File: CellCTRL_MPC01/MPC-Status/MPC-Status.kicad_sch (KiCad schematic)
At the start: 38 parts, among them J1 Programming, J2 I2C, J3 Reset, U1 ATtiny202-SS

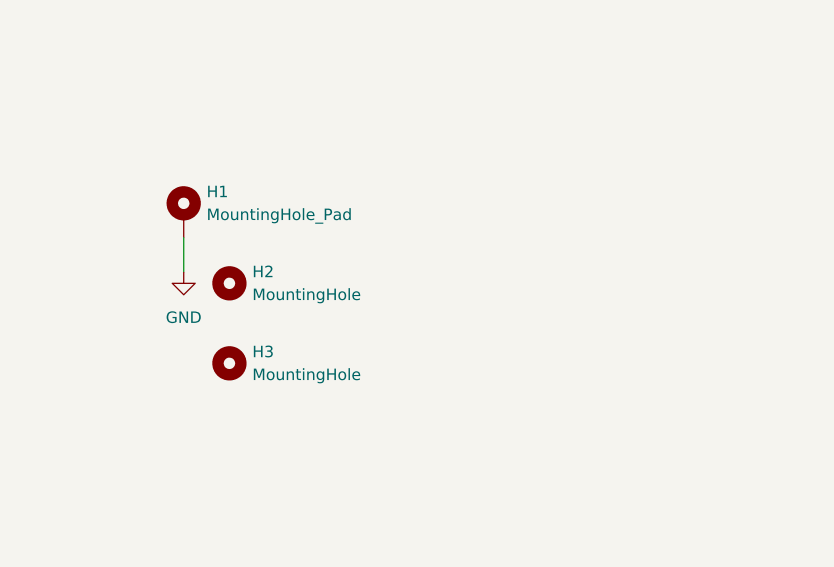
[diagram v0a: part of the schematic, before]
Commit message: Fertig V0.1_Status
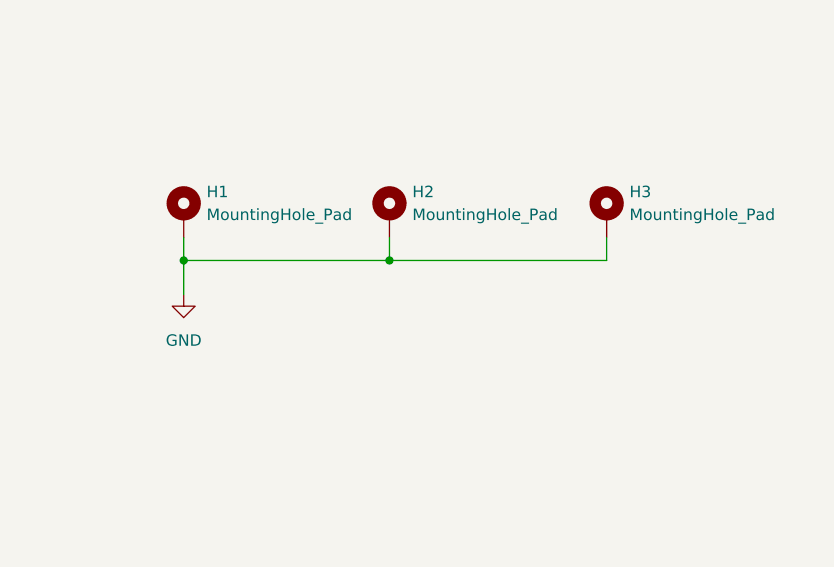
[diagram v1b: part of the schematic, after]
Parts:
- removed H2, H3: MountingHole, MountingHole:MountingHole_3.2mm_M3_DIN965, symbol Mechanical:MountingHole
- added H2, H3: MountingHole_Pad, MountingHole:MountingHole_3.2mm_M3_DIN965_Pad, symbol Mechanical:MountingHole_Pad
- J2: footprint Connector_JST:JST_EH_B4B-EH-A_1x04_P2.50mm_Vertical -> Connector_JST:JST_XH_B4B-XH-A_1x04_P2.50mm_Vertical
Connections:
- net GND: now also H2.1, H3.1
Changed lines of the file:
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@@
 	)
 	(junction
+		(at 227.33 93.98)
+		(diameter 0)
+		(color 0 0 0 0)
+	)
+	(junction
 		(at 82.55 148.59)
 		(diameter 0)
@@
 	)
 	(junction
+		(at 204.47 93.98)
+		(diameter 0)
+		(color 0 0 0 0)
+	)
+	(junction
 		(at 152.4 34.29)
 		(diameter 0)
@@
 	(wire
 		(pts
+			(xy 251.46 93.98) (xy 227.33 93.98)
+		)
+		(stroke
+			(width 0)
+			(type default)
+		)
+	)
+	(wire
+		(pts
 			(xy 57.15 135.89) (xy 62.23 135.89)
 		)
@@
 	(wire
 		(pts
+			(xy 251.46 91.44) (xy 251.46 93.98)
+		)
+		(stroke
+			(width 0)
+			(type default)
+		)
+	)
+	(wire
+		(pts
 			(xy 62.23 133.35) (xy 62.23 135.89)
 		)
@@
 	(wire
 		(pts
+			(xy 227.33 93.98) (xy 204.47 93.98)
+		)
+		(stroke
+			(width 0)
+			(type default)
+		)
+	)
+	(wire
+		(pts
 			(xy 160.02 46.99) (xy 167.64 46.99)
 		)
@@
 	(wire
 		(pts
-			(xy 204.47 91.44) (xy 204.47 95.25)
+			(xy 227.33 91.44) (xy 227.33 93.98)
+		)
+		(stroke
+			(width 0)
+			(type default)
+		)
+	)
+	(wire
+		(pts
+			(xy 204.47 91.44) (xy 204.47 93.98)
 		)
 		(stroke
@@
 	(wire
 		(pts
+			(xy 204.47 93.98) (xy 204.47 97.79)
+		)
+		(stroke
+			(width 0)
+			(type default)
+		)
+	)
+	(wire
+		(pts
 			(xy 198.12 39.37) (xy 198.12 34.29)
 		)
@@
 	)
 	(symbol
-		(lib_id "Mechanical:MountingHole")
-		(at 209.55 105.41 0)
-		(unit 1)
-		(exclude_from_sim no)
-		(in_bom no)
-		(on_board yes)
-		(dnp no)
-		(fields_autoplaced yes)
-		(property "Reference" "H3"
-			(at 212.09 104.1399 0)
-			(effects
-				(font
-					(size 1.27 1.27)
-				)
-				(justify left)
-			)
-		)
-		(property "Value" "MountingHole"
-			(at 212.09 106.6799 0)
-			(effects
-				(font
-					(size 1.27 1.27)
-				)
-				(justify left)
-			)
-		)
-		(property "Footprint" "MountingHole:MountingHole_3.2mm_M3_DIN965"
-			(at 209.55 105.41 0)
-			(effects
-				(font
-					(size 1.27 1.27)
-				)
-				(hide yes)
-			)
-		)
-		(property "Datasheet" "~"
-			(at 209.55 105.41 0)
-			(effects
-				(font
-					(size 1.27 1.27)
-				)
-				(hide yes)
-			)
-		)
-		(property "Description" "Mounting Hole without connection"
-			(at 209.55 105.41 0)
-			(effects
-				(font
-					(size 1.27 1.27)
-				)
-				(hide yes)
-			)
-		)
-		(instances
-			(project "MPC-Status"
-				(path "/6205391b-a61f-4e60-b73e-3eadab0d3997"
-					(reference "H3")
-					(unit 1)
-				)
-			)
-		)
-	)
-	(symbol
 		(lib_id "power:GND")
 		(at 152.4 20.32 180)
@@
 	)
 	(symbol
-		(lib_id "Mechanical:MountingHole")
-		(at 209.55 96.52 0)
-		(unit 1)
-		(exclude_from_sim no)
-		(in_bom no)
-		(on_board yes)
-		(dnp no)
-		(fields_autoplaced yes)
-		(property "Reference" "H2"
-			(at 212.09 95.2499 0)
-			(effects
-				(font
-					(size 1.27 1.27)
-				)
-				(justify left)
-			)
-		)
-		(property "Value" "MountingHole"
-			(at 212.09 97.7899 0)
-			(effects
-				(font
-					(size 1.27 1.27)
-				)
-				(justify left)
-			)
-		)
-		(property "Footprint" "MountingHole:MountingHole_3.2mm_M3_DIN965"
-			(at 209.55 96.52 0)
-			(effects
-				(font
-					(size 1.27 1.27)
-				)
-				(hide yes)
-			)
-		)
-		(property "Datasheet" "~"
-			(at 209.55 96.52 0)
-			(effects
-				(font
-					(size 1.27 1.27)
-				)
-				(hide yes)
-			)
-		)
-		(property "Description" "Mounting Hole without connection"
-			(at 209.55 96.52 0)
-			(effects
-				(font
-					(size 1.27 1.27)
-				)
-				(hide yes)
-			)
-		)
-		(instances
-			(project ""
-				(path "/6205391b-a61f-4e60-b73e-3eadab0d3997"
-					(reference "H2")
-					(unit 1)
-				)
-			)
-		)
-	)
-	(symbol
 		(lib_id "Device:C")
 		(at 175.26 26.67 180)
@@
 	(symbol
 		(lib_id "power:GND")
-		(at 204.47 95.25 0)
+		(at 204.47 97.79 0)
 		(unit 1)
 		(exclude_from_sim no)
@@
 		(fields_autoplaced yes)
 		(property "Reference" "#PWR030"
-			(at 204.47 101.6 0)
+			(at 204.47 104.14 0)
 			(effects
 				(font
@@
 		)
 		(property "Value" "GND"
-			(at 204.47 100.33 0)
+			(at 204.47 102.87 0)
 			(effects
 				(font
@@
 		)
 		(property "Footprint" ""
-			(at 204.47 95.25 0)
+			(at 204.47 97.79 0)
 			(effects
 				(font
@@
 		)
 		(property "Datasheet" ""
-			(at 204.47 95.25 0)
+			(at 204.47 97.79 0)
 			(effects
 				(font
@@
 		)
 		(property "Description" "Power symbol creates a global label with name \"GND\" , ground"
-			(at 204.47 95.25 0)
+			(at 204.47 97.79 0)
 			(effects
 				(font
@@
 	)
 	(symbol
+		(lib_id "Mechanical:MountingHole_Pad")
+		(at 251.46 88.9 0)
+		(unit 1)
+		(exclude_from_sim no)
+		(in_bom no)
+		(on_board yes)
+		(dnp no)
+		(fields_autoplaced yes)
+		(property "Reference" "H3"
+			(at 254 86.3599 0)
+			(effects
+				(font
+					(size 1.27 1.27)
+				)
+				(justify left)
+			)
+		)
+		(property "Value" "MountingHole_Pad"
+			(at 254 88.8999 0)
+			(effects
+				(font
+					(size 1.27 1.27)
+				)
+				(justify left)
+			)
+		)
+		(property "Footprint" "MountingHole:MountingHole_3.2mm_M3_DIN965_Pad"
+			(at 251.46 88.9 0)
+			(effects
+				(font
+					(size 1.27 1.27)
+				)
+				(hide yes)
+			)
+		)
+		(property "Datasheet" "~"
+			(at 251.46 88.9 0)
+			(effects
+				(font
+					(size 1.27 1.27)
+				)
+				(hide yes)
+			)
+		)
+		(property "Description" "Mounting Hole with connection"
+			(at 251.46 88.9 0)
+			(effects
+				(font
+					(size 1.27 1.27)
+				)
+				(hide yes)
+			)
+		)
+		(pin "1"
+		)
+		(instances
+			(project "MPC-Status"
+				(path "/6205391b-a61f-4e60-b73e-3eadab0d3997"
+					(reference "H3")
+					(unit 1)
+				)
+			)
+		)
+	)
+	(symbol
 		(lib_id "Device:C")
 		(at 129.54 26.67 180)
@@
 			)
 		)
-		(property "Footprint" "Connector_JST:JST_EH_B4B-EH-A_1x04_P2.50mm_Vertical"
+		(property "Footprint" "Connector_JST:JST_XH_B4B-XH-A_1x04_P2.50mm_Vertical"
 			(at 156.21 185.42 0)
 			(effects
@@
 					(unit 1)
 				)
+			)
+		)
+	)
+	(symbol
+		(lib_id "Mechanical:MountingHole_Pad")
+		(at 227.33 88.9 0)
+		(unit 1)
+		(exclude_from_sim no)
+		(in_bom no)
+		(on_board yes)
+		(dnp no)
+		(fields_autoplaced yes)
+		(property "Reference" "H2"
+			(at 229.87 86.3599 0)
+			(effects
+				(font
+					(size 1.27 1.27)
+				)
+				(justify left)
+			)
+		)
+		(property "Value" "MountingHole_Pad"
+			(at 229.87 88.8999 0)
+			(effects
+				(font
+					(size 1.27 1.27)
+				)
+				(justify left)
+			)
+		)
+		(property "Footprint" "MountingHole:MountingHole_3.2mm_M3_DIN965_Pad"
+			(at 227.33 88.9 0)
+			(effects
+				(font
+					(size 1.27 1.27)
+				)
+				(hide yes)
+			)
+		)
+		(property "Datasheet" "~"
+			(at 227.33 88.9 0)
+			(effects
+				(font
+					(size 1.27 1.27)
+				)
+				(hide yes)
+			)
+		)
+		(property "Description" "Mounting Hole with connection"
+			(at 227.33 88.9 0)
+			(effects
+				(font
+					(size 1.27 1.27)
+				)
+				(hide yes)
+			)
+		)
+		(pin "1"
+		)
+		(instances
+			(project "MPC-Status"
+				(path "/6205391b-a61f-4e60-b73e-3eadab0d3997"
+					(reference "H2")
+					(unit 1)
+				)
